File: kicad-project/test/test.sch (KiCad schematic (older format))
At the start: 20 parts

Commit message: Kicad начало 2 лабы
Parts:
- BF1, C1, C2, C3, C4: footprint (none) -> Capacitors_SMD:C_0805
- D1: footprint (none) -> SMD_Packages:SOIC-8-N
- R1, R2, R3, R4, R6, R7, R8, R9: footprint (none) -> Resistors_SMD:R_0805
- VD1, VD2: footprint (none) -> Diodes_SMD:D_0805
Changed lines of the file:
@@
 F 0 "R4" V 1180 950 50  0000 C CNN
 F 1 "10K" V 1100 950 50  0000 C CNN
-F 2 "" V 1030 950 50  0001 C CNN
+F 2 "Resistors_SMD:R_0805" V 1030 950 50  0001 C CNN
 F 3 "" H 1100 950 50  0001 C CNN
 	1    1100 950
@@
 F 0 "R1" V 880 1450 50  0000 C CNN
 F 1 "220K" V 800 1450 50  0000 C CNN
-F 2 "" V 730 1450 50  0001 C CNN
+F 2 "Resistors_SMD:R_0805" V 730 1450 50  0001 C CNN
 F 3 "" H 800 1450 50  0001 C CNN
 	1    800  1450
@@
 F 0 "D1" H 3150 2100 60  0000 C CNN
 F 1 "КР1436АП1" H 3700 2100 60  0000 C CNN
-F 2 "" H 3500 2300 60  0001 C CNN
+F 2 "SMD_Packages:SOIC-8-N" H 3500 2300 60  0001 C CNN
 F 3 "" H 3500 2300 60  0001 C CNN
 	1    3500 1450
@@
 F 0 "C1" H 2125 1050 50  0000 L CNN
 F 1 "1мкФ" H 2125 850 50  0000 L CNN
-F 2 "" H 2138 800 12  0001 C CNN
+F 2 "Capacitors_SMD:C_0805" H 2138 800 12  0001 C CNN
 F 3 "" H 2100 950 39  0001 C CNN
 	1    2100 950
@@
 F 0 "R2" V 880 2800 50  0000 C CNN
 F 1 "1M" V 800 2800 50  0000 C CNN
-F 2 "" V 730 2800 50  0001 C CNN
+F 2 "Resistors_SMD:R_0805" V 730 2800 50  0001 C CNN
 F 3 "" H 800 2800 50  0001 C CNN
 	1    800  2800
@@
 F 0 "R3" V 1330 2800 50  0000 C CNN
 F 1 "100K" V 1250 2800 50  0000 C CNN
-F 2 "" V 1180 2800 50  0001 C CNN
+F 2 "Resistors_SMD:R_0805" V 1180 2800 50  0001 C CNN
 F 3 "" H 1250 2800 50  0001 C CNN
 	1    1250 2800
@@
 F 0 "R6" V 1780 2800 50  0000 C CNN
 F 1 "22K" V 1700 2800 50  0000 C CNN
-F 2 "" V 1630 2800 50  0001 C CNN
+F 2 "Resistors_SMD:R_0805" V 1630 2800 50  0001 C CNN
 F 3 "" H 1700 2800 50  0001 C CNN
 	1    1700 2800
@@
 F 0 "VD2" H 2150 1750 50  0000 C CNN
 F 1 "КД522" H 2150 1550 50  0000 C CNN
-F 2 "" H 2150 1650 50  0001 C CNN
+F 2 "Diodes_SMD:D_0805" H 2150 1650 50  0001 C CNN
 F 3 "" H 2150 1650 50  0001 C CNN
 	1    2150 1650
@@
 F 0 "VD1" H 1850 1550 50  0000 C CNN
 F 1 "КД522" H 1850 1350 50  0000 C CNN
-F 2 "" H 1850 1450 50  0001 C CNN
+F 2 "Diodes_SMD:D_0805" H 1850 1450 50  0001 C CNN
 F 3 "" H 1850 1450 50  0001 C CNN
 	1    1850 1450
@@
 F 0 "R7" V 2580 1850 50  0000 C CNN
 F 1 "R" V 2500 1850 50  0000 C CNN
-F 2 "" V 2430 1850 50  0001 C CNN
+F 2 "Resistors_SMD:R_0805" V 2430 1850 50  0001 C CNN
 F 3 "" H 2500 1850 50  0001 C CNN
 	1    2500 1850
@@
 F 0 "C2" H 2375 2200 50  0000 L CNN
 F 1 "0,47мкФ" H 2375 2000 50  0000 L CNN
-F 2 "" H 2388 1950 50  0001 C CNN
+F 2 "Capacitors_SMD:C_0805" H 2388 1950 50  0001 C CNN
 F 3 "" H 2350 2100 50  0001 C CNN
 	1    2350 2100
@@
 F 0 "R8" V 2730 2800 50  0000 C CNN
 F 1 "300K" V 2650 2800 50  0000 C CNN
-F 2 "" V 2580 2800 50  0001 C CNN
+F 2 "Resistors_SMD:R_0805" V 2580 2800 50  0001 C CNN
 F 3 "" H 2650 2800 50  0001 C CNN
 	1    2650 2800
@@
 F 0 "R9" V 4580 1650 50  0000 C CNN
 F 1 "120K" V 4500 1650 50  0000 C CNN
-F 2 "" V 4430 1650 50  0001 C CNN
+F 2 "Resistors_SMD:R_0805" V 4430 1650 50  0001 C CNN
 F 3 "" H 4500 1650 50  0001 C CNN
 	1    4500 1650
@@
 F 0 "C4" H 4975 1900 50  0000 L CNN
 F 1 "10нФ" H 4975 1700 50  0000 L CNN
-F 2 "" H 4988 1650 50  0001 C CNN
+F 2 "Capacitors_SMD:C_0805" H 4988 1650 50  0001 C CNN
 F 3 "" H 4950 1800 50  0001 C CNN
 	1    4950 1800
@@
 F 0 "C3" H 4925 950 50  0000 L CNN
 F 1 "0,22мкФ" H 4925 750 50  0000 L CNN
-F 2 "" H 4938 700 50  0001 C CNN
+F 2 "Capacitors_SMD:C_0805" H 4938 700 50  0001 C CNN
 F 3 "" H 4900 850 50  0001 C CNN
 	1    4900 850
@@
 F 0 "BF1" H 5550 1200 60  0000 C CNN
 F 1 "ЗП-25" H 5600 1100 60  0000 C CNN
-F 2 "" H 5400 1150 60  0001 C CNN
+F 2 "Capacitors_SMD:C_0805" H 5400 1150 60  0001 C CNN
 F 3 "" H 5400 1150 60  0001 C CNN
 	1    5400 1150

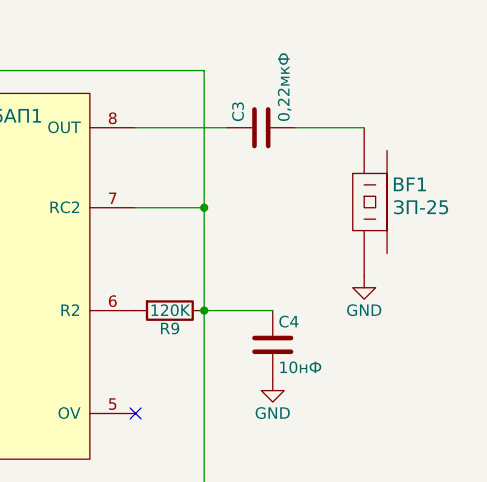
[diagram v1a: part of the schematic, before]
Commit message: kicad 2 лаба
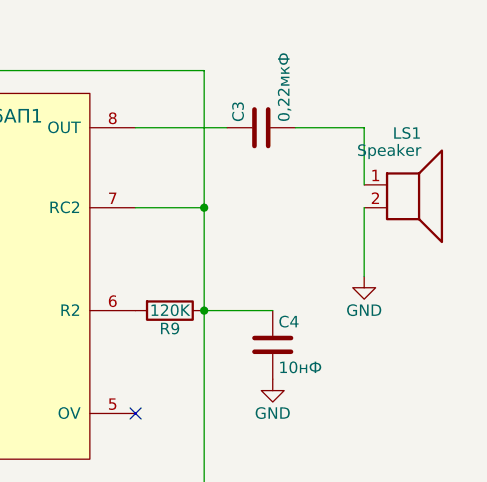
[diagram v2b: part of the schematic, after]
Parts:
- removed BF1: ЗП-25, Capacitors_SMD:C_0805, symbol ЗП-25
- added LS1: Speaker, Battery_Holders:Seiko_MS621F, symbol Speaker
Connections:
- net GND: now also LS1.2
- net at C3.2: now also LS1.1
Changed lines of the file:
@@
 Wire Wire Line
 	4350 850  4750 850
-$Comp
-L ЗП-25 BF1
-U 1 1 5A04BC1B
-P 5400 1150
-F 0 "BF1" H 5550 1200 60  0000 C CNN
-F 1 "ЗП-25" H 5600 1100 60  0000 C CNN
-F 2 "Capacitors_SMD:C_0805" H 5400 1150 60  0001 C CNN
-F 3 "" H 5400 1150 60  0001 C CNN
-	1    5400 1150
-	1    0    0    -1
-$EndComp
 Wire Wire Line
 	5350 850  5050 850
@@
 Wire Wire Line
 	600  1100 600  1200
+$Comp
+L Speaker LS1
+U 1 1 5A0F908D
+P 5550 1100
+F 0 "LS1" H 5600 1325 50  0000 R CNN
+F 1 "Speaker" H 5600 1250 50  0000 R CNN
+F 2 "Battery_Holders:Seiko_MS621F" H 5550 900 50  0001 C CNN
+F 3 "" H 5540 1050 50  0001 C CNN
+	1    5550 1100
+	1    0    0    -1
+$EndComp
+Wire Wire Line
+	5350 850  5350 1100
+Wire Wire Line
+	5350 1200 5350 1500
 $EndSCHEMATC
